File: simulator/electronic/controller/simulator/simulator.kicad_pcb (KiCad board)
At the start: 2 copper layers, 151 x 92.5 mm, 45 parts, among them J1 Conn_01x04_Socket, J2 Conn_01x04_Socket, J3 Conn_01x04_Socket, J4 Conn_01x04_Socket, J5 Conn_01x04_Socket, J6 Conn_01x04_Socket, J7 Conn_01x04_Socket, J8 Conn_01x04_Socket, U1 ESP32 D1 Mini

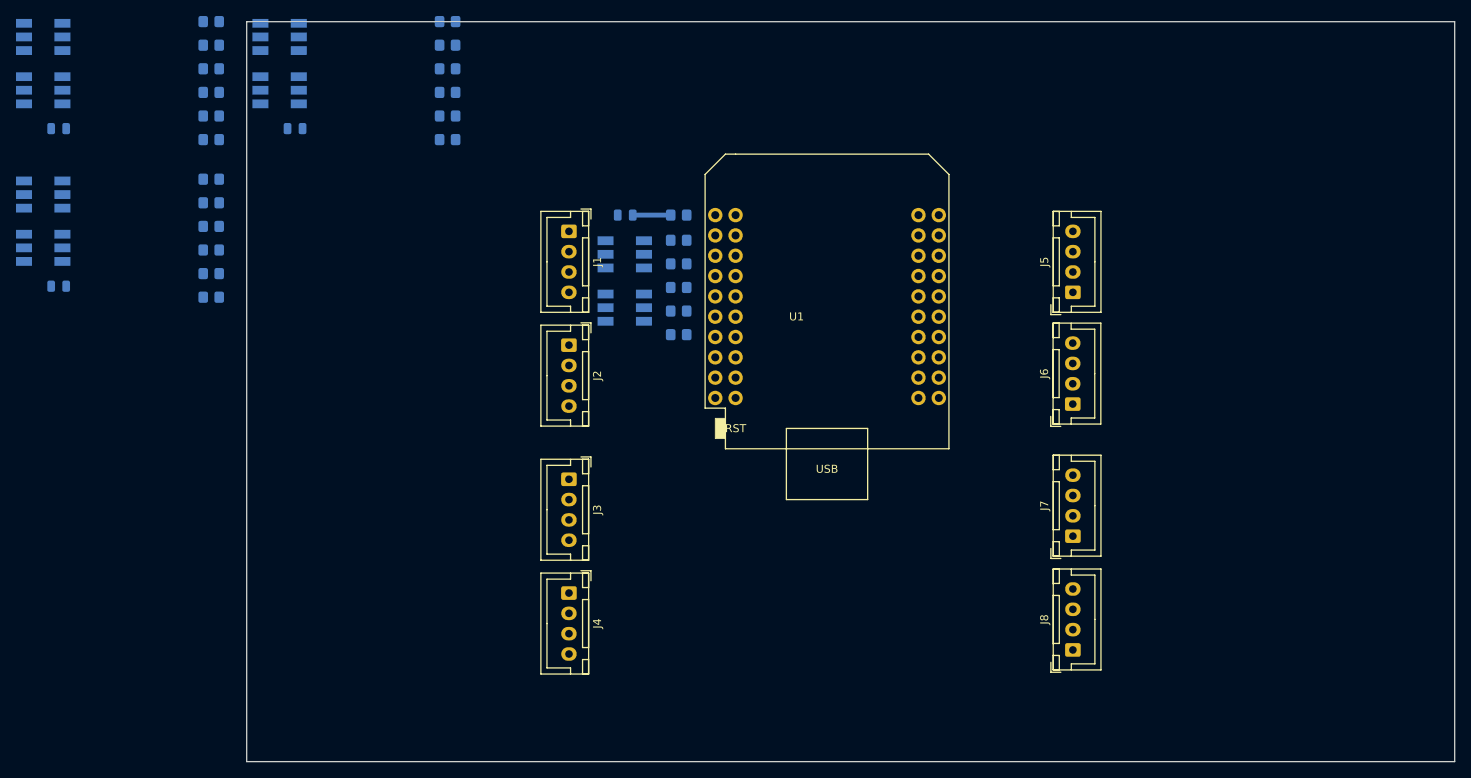
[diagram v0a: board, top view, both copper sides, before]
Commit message: update simulator
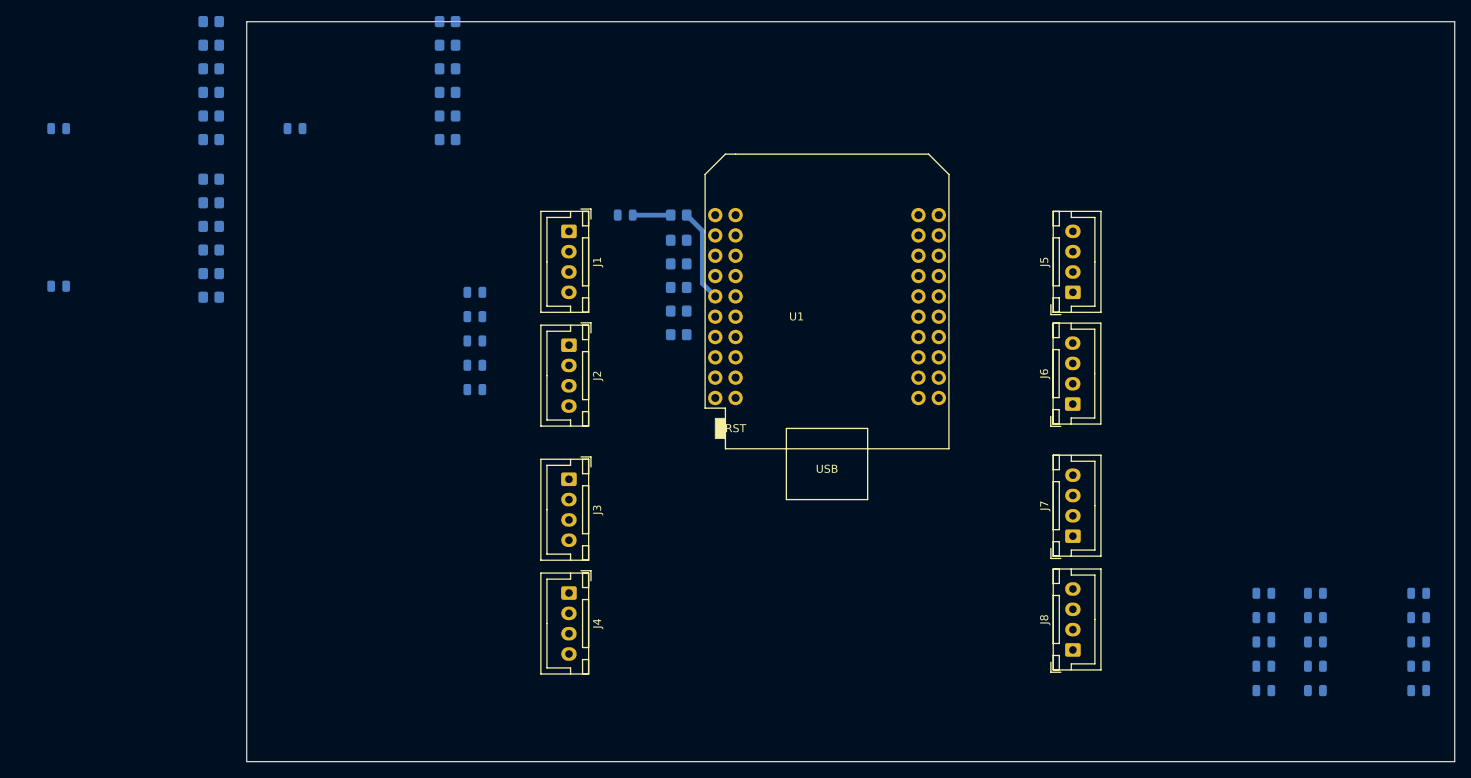
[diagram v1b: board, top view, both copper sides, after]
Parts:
- added D10: LED_CENTER, LED_SMD:LED_0805_2012Metric, B.Cu at (200.1, 128.5)
- added D14: LED_TOP, LED_SMD:LED_0805_2012Metric, B.Cu at (219.5, 122.5)
- added D15: LED_UP, LED_SMD:LED_0805_2012Metric, B.Cu at (219.5, 125.5)
- added D16: LED_CENTER, LED_SMD:LED_0805_2012Metric, B.Cu at (219.5, 128.5)
- added D17: LED_BTM, LED_SMD:LED_0805_2012Metric, B.Cu at (219.5, 131.6)
- added D18: LED_DOWN, LED_SMD:LED_0805_2012Metric, B.Cu at (219.5, 134.6)
- added D20: LED_TOP, LED_SMD:LED_0805_2012Metric, B.Cu at (206.6, 122.5)
- added D21: LED_UP, LED_SMD:LED_0805_2012Metric, B.Cu at (206.6, 125.5)
- added D22: LED_CENTER, LED_SMD:LED_0805_2012Metric, B.Cu at (206.6, 128.5)
- added D23: LED_BTM, LED_SMD:LED_0805_2012Metric, B.Cu at (206.6, 131.6)
- added D24: LED_DOWN, LED_SMD:LED_0805_2012Metric, B.Cu at (206.6, 134.6)
- added D4: LED_CENTER, LED_SMD:LED_0805_2012Metric, B.Cu at (101.5, 90.9)
- D11, D5: value LED_DIR -> LED_BTM; footprint LED_SMD:LED_RGB_5050-6 -> LED_SMD:LED_0805_2012Metric
- D12, D6: value LED_SW -> LED_DOWN; footprint LED_SMD:LED_RGB_5050-6 -> LED_SMD:LED_0805_2012Metric
- D2, D8: value LED_DIR -> LED_TOP; footprint LED_SMD:LED_RGB_5050-6 -> LED_SMD:LED_0805_2012Metric
- D3, D9: value LED_SW -> LED_UP; footprint LED_SMD:LED_RGB_5050-6 -> LED_SMD:LED_0805_2012Metric
- moved D11 171.7 mm to (200.1, 131.6)
- moved D12 170.0 mm to (200.1, 134.6)
- moved D8 141.3 mm to (200.1, 122.5)
- moved D9 139.6 mm to (200.1, 125.5)
- moved D5 58.0 mm to (101.5, 94.0)
- moved D6 56.8 mm to (101.5, 97.0)
- moved D2 19.3 mm to (101.5, 84.8)
- moved D3 18.8 mm to (101.5, 87.9)
- turned R2 to 0 degrees
- turned R3 to 0 degrees
- turned R4 to 0 degrees
- turned R5 to 0 degrees
- turned R6 to 0 degrees
- renumbered D7 to D13, D10 to D19, D4 to D7, R11 to R10, R12 to R11, R10 to R12, R15 to R14, R14 to R15, R17 to R16, R18 to R17, R16 to R18, R7 to R2, R21 to R20, R20 to R21, R23 to R22, R24 to R23, R22 to R24, R2 to R3, R6 to R4, R3 to R6, R4 to R7, R9 to R8, R8 to R9
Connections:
- D1 pad 2: unconnected-(D1-A-Pad2) -> Net-(D1-A)
- D11 pad 1: unconnected-(D11-RK-Pad1) -> Net-(D11-K)
- D12 pad 1: 3V3 -> Net-(D12-K)
- D2 pad 1: unconnected-(D2-RK-Pad1) -> Net-(D2-K)
- D3 pad 1: 3V3 -> GND
- D3 pad 2: 3V3 -> Net-(D3-A)
- D5 pad 1: unconnected-(D5-RK-Pad1) -> Net-(D5-K)
- D6 pad 1: 3V3 -> Net-(D6-K)
- D8 pad 1: unconnected-(D8-RK-Pad1) -> Net-(D8-K)
- D9 pad 1: 3V3 -> GND
- D9 pad 2: 3V3 -> Net-(D9-A)
- R1 pad 1: unconnected-(D1-A-Pad2) -> Net-(D1-A)
- R10 pad 1: Net-(D6-GA) -> Net-(D10-K)
- R11 pad 1: Net-(D6-BA) -> Net-(D11-K)
- R12 pad 1: Net-(D5-GA) -> Net-(D12-K)
- R14 pad 1: Net-(D9-RA) -> Net-(D14-K)
- R15 pad 1: Net-(D8-BA) -> Net-(D15-A)
- R16 pad 1: Net-(D9-GA) -> Net-(D16-K)
- R17 pad 1: Net-(D9-BA) -> Net-(D17-K)
- R18 pad 1: Net-(D8-GA) -> Net-(D18-K)
- R2 pad 1: Net-(D3-RA) -> Net-(D2-K)
- R20 pad 1: Net-(D12-RA) -> Net-(D20-K)
- R21 pad 1: Net-(D11-BA) -> Net-(D21-A)
- R22 pad 1: Net-(D12-GA) -> Net-(D22-K)
- R23 pad 1: Net-(D12-BA) -> Net-(D23-K)
- R24 pad 1: Net-(D11-GA) -> Net-(D24-K)
- R3 pad 1: Net-(D2-BA) -> Net-(D3-A)
- R4 pad 1: Net-(D3-GA) -> Net-(D4-K)
- R5 pad 1: Net-(D3-BA) -> Net-(D5-K)
- R6 pad 1: Net-(D2-GA) -> Net-(D6-K)
- R8 pad 1: Net-(D6-RA) -> Net-(D8-K)
- R9 pad 1: Net-(D5-BA) -> Net-(D9-A)
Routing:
- net /connection/PULSE: track 0.00 -> 11.6 mm
- net unconnected-(D1-A-Pad2): track 4.75 -> 0.00 mm
- net Net-(D1-A): track 0.00 -> 4.75 mm

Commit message: update simulator
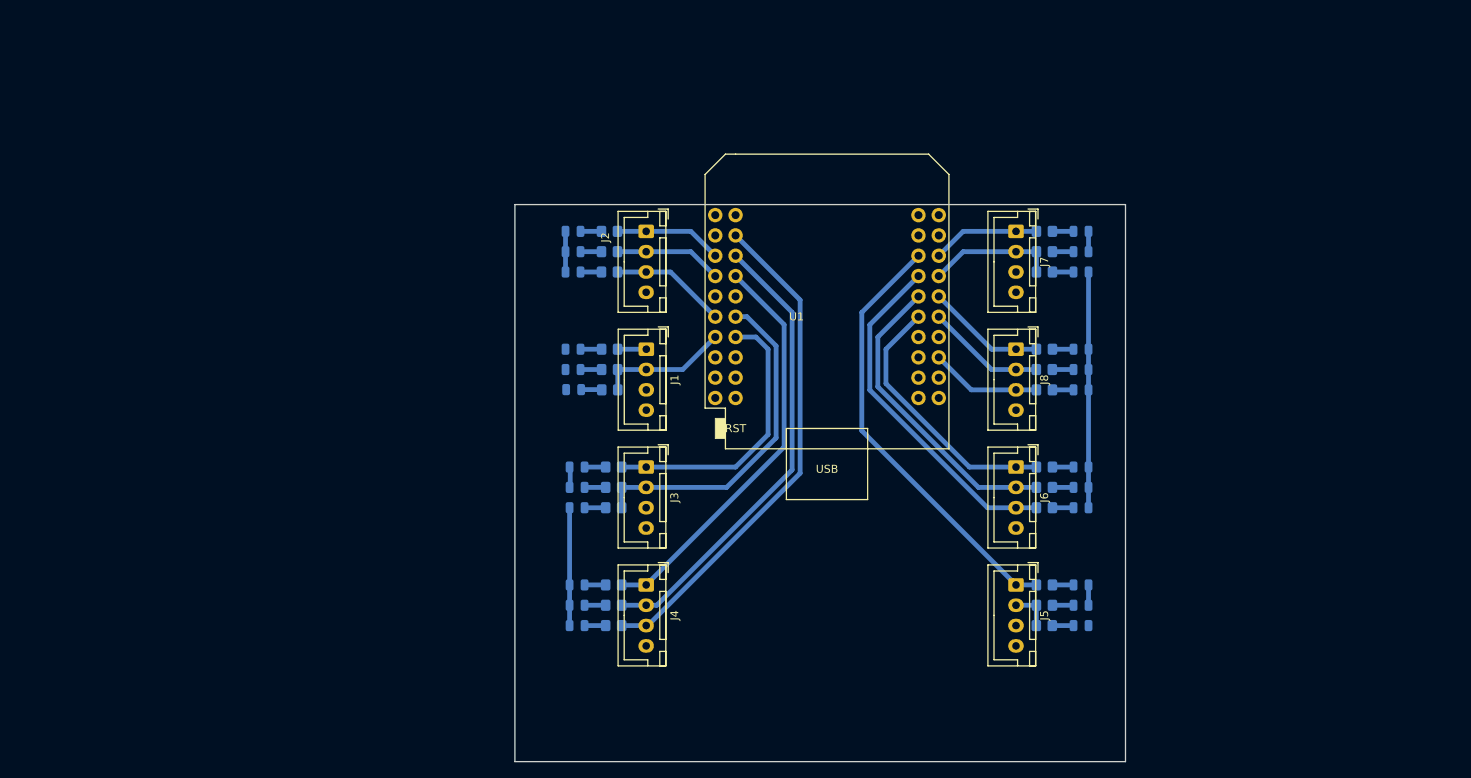
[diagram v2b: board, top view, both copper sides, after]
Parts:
- moved D19 128.4 mm to (177.3, 77.2)
- moved D13 113.6 mm to (177.3, 121.4)
- moved R22 109.9 mm to (172.7, 91.9)
- moved R23 108.9 mm to (172.7, 94.5)
- moved R24 108.8 mm to (172.7, 97.0)
- moved R19 107.4 mm to (172.7, 77.2)
- moved R20 107.3 mm to (172.7, 79.8)
- moved R21 106.5 mm to (172.7, 82.3)
- moved R13 102.6 mm to (172.7, 121.4)
- moved R14 102.3 mm to (172.7, 124.0)
- moved R15 100.0 mm to (172.7, 126.5)
- moved R16 89.7 mm to (172.7, 106.7)
- moved D9 88.8 mm to (114.3, 111.8)
- moved R17 87.9 mm to (172.7, 109.2)
- moved R18 87.7 mm to (172.7, 111.8)
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- renumbered D8 to D10, D10 to D11, D11 to D12, D15 to D14, D18 to D15, D14 to D16, D16 to D17, D17 to D18, D3 to D2, D21 to D20, D24 to D21, D20 to D22, D22 to D23, D23 to D24, D6 to D3, D2 to D4, D4 to D5, D5 to D6, D9 to D8, D12 to D9, R8 to R10, R10 to R11, R11 to R12, R15 to R14, R18 to R15, R14 to R16, R16 to R17, R17 to R18, R3 to R2, R21 to R20, R24 to R21, R20 to R22, R22 to R23, R23 to R24, R6 to R3, R2 to R4, R4 to R5, R5 to R6, R9 to R8, R12 to R9
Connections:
- U1 pad 24: /connection2/SW_BOTTOM -> /connection2/DIR
- U1 pad 27: /connection2/DIR -> /connection2/SW_BOTTOM
- U1 pad 29: /connection2/SW_TOP -> /connection2/SW_CENTER
- U1 pad 31: /connection2/SW_CENTER -> /connection2/SW_TOP
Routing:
- net /connection1/SW_BOTTOM: track 0.00 -> 63.3 mm
- net /connection1/SW_CENTER: track 0.00 -> 58.0 mm
- net /connection2/PULSE: track 0.00 -> 54.6 mm
- net /connection1/SW_TOP: track 0.00 -> 51.3 mm
- net 3V3: track 0.00 -> 49.3 mm
- net /connection2/SW_BOTTOM: track 0.00 -> 43.7 mm
- net /connection1/DIR: track 0.00 -> 42.5 mm
- net /connection2/SW_CENTER: track 0.00 -> 38.4 mm
- net /connection1/PULSE: track 0.00 -> 35.4 mm
- net /connection2/SW_TOP: track 0.00 -> 33.2 mm
- net /connection/DIR: track 0.00 -> 16.4 mm
- net /connection3/DIR: track 0.00 -> 16.0 mm
- net /connection3/SW_TOP: track 0.00 -> 14.9 mm
- net /connection3/SW_CENTER: track 0.00 -> 14.9 mm
- net /connection/SW_BOTTOM: track 0.00 -> 14.5 mm
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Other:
- board size 151 x 92.5 mm -> 76.3 x 69.6 mm
